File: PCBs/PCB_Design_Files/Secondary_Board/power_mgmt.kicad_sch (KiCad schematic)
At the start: 19 parts, among them Q3 MMBT3904, Q4 MMBT3904, U1 TPS61023DRLR, U2 TLV9101IDCKR

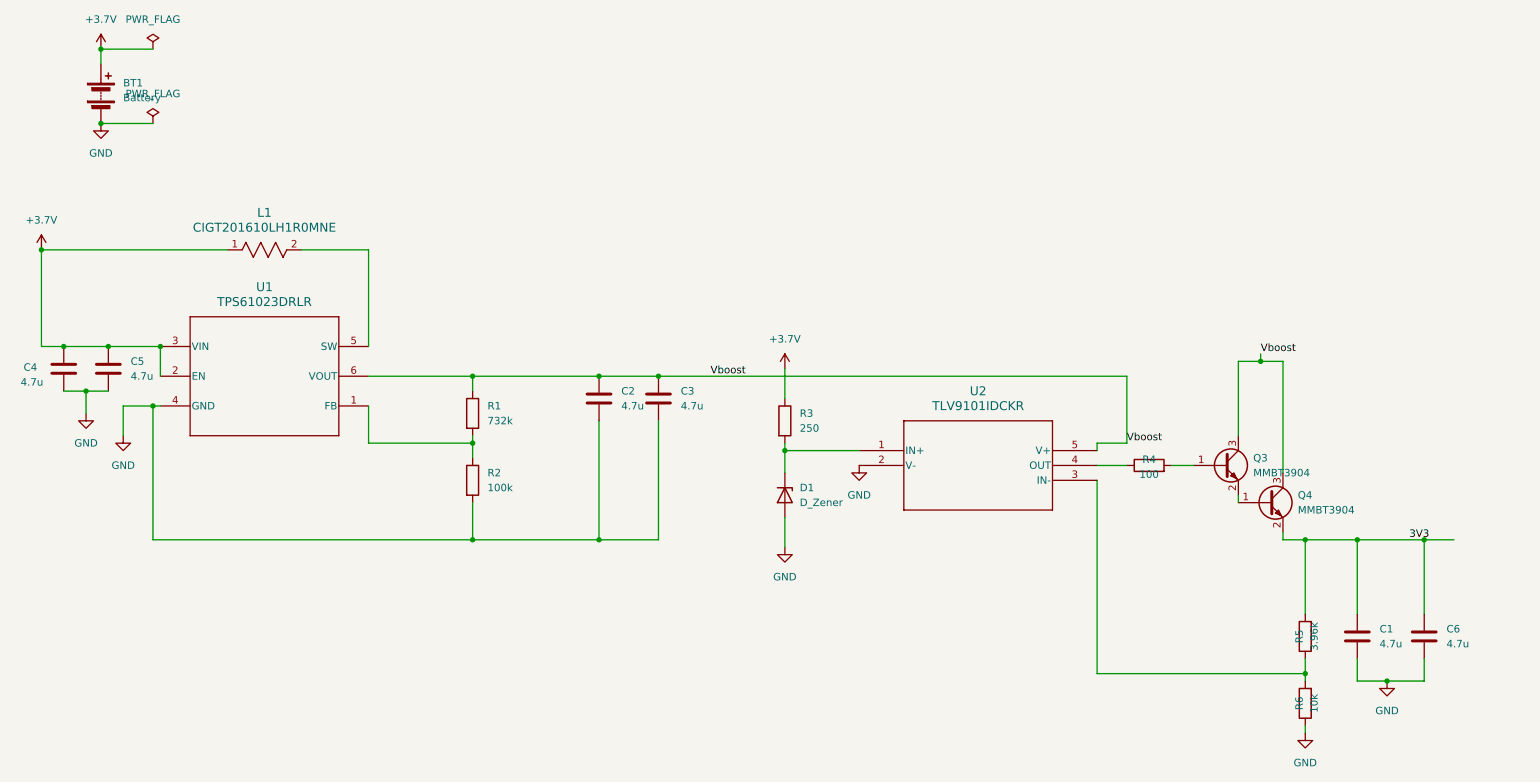
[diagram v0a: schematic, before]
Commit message: footprint update
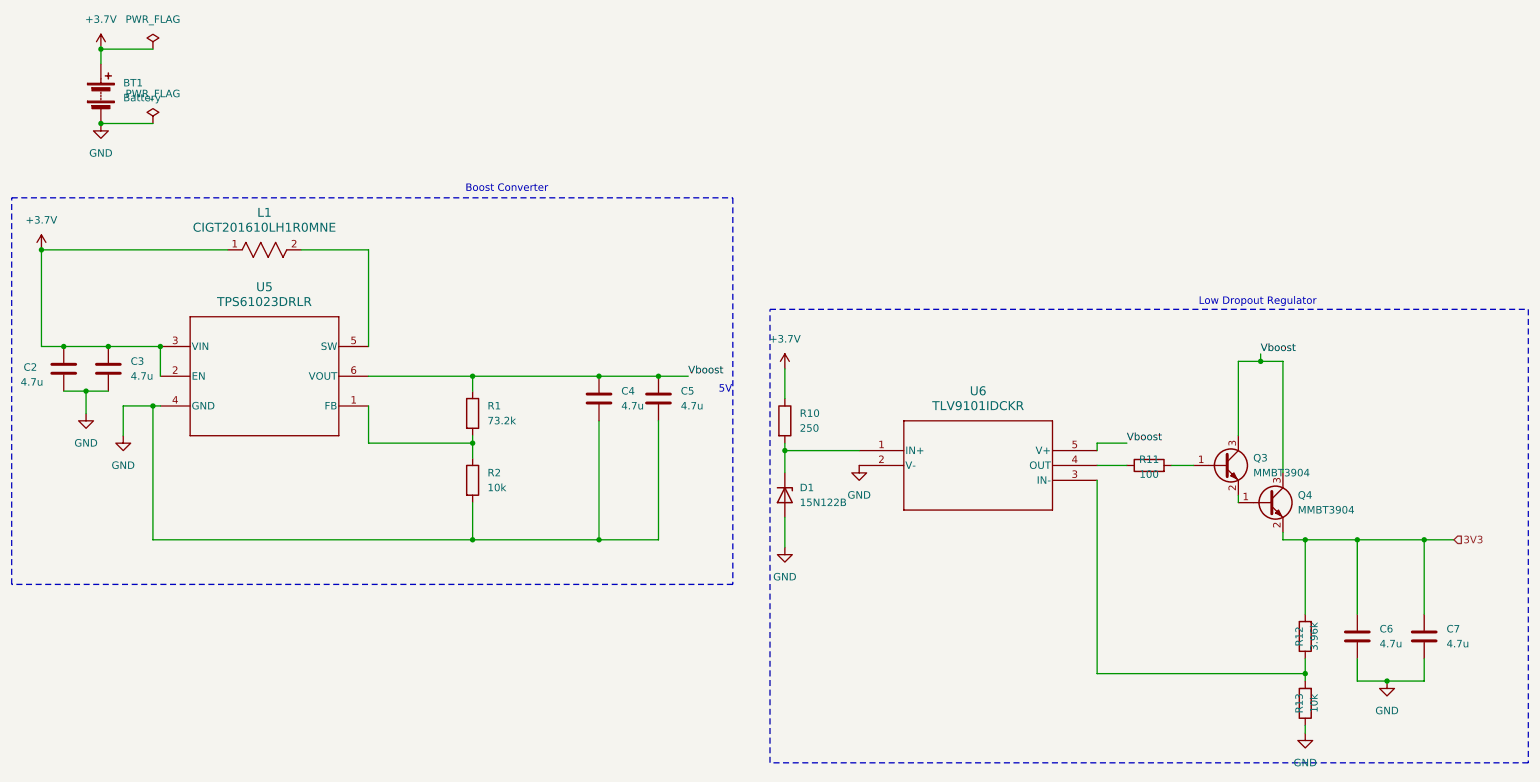
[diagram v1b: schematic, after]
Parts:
- BT1: footprint (none) -> Diode_THT:D_DO-35_SOD27_P7.62mm_Horizontal
- D1: value D_Zener -> 15N122B; footprint (none) -> Diode_THT:D_DO-35_SOD27_P7.62mm_Horizontal
- L1: footprint RES_CIGT201610_SAM -> Project Footprints:RES_CIGT201610_SAM
- Q3, Q4: footprint Package_TO_SOT_SMD:SOT-23 -> Project Footprints:SOT23_FAS
- R1: value 732k -> 73.2k; footprint Resistor_SMD:R_0201_0603Metric -> Project Footprints:0603_resistor
- R10: renamed from R3; footprint Resistor_SMD:R_0201_0603Metric -> Project Footprints:0603_resistor
- R11: renamed from R4; footprint Resistor_SMD:R_0201_0603Metric -> Project Footprints:0603_resistor
- R12: renamed from R5; footprint Resistor_SMD:R_0201_0603Metric -> Project Footprints:0603_resistor
- R13: renamed from R6; footprint Resistor_SMD:R_0201_0603Metric -> Project Footprints:0603_resistor
- R2: value 100k -> 10k; footprint (none) -> Project Footprints:0603_resistor
- U6: renamed from U2; footprint SC70-5_DCK_TEX -> Project Footprints:SC70-5_DCK_TEX
- renumbered C4 to C2, C5 to C3, C2 to C4, C3 to C5, C1 to C6, C6 to C7, U1 to U5
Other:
- note added: "5V"
- note added: "Boost Converter"
- note added: "Low Dropout Regulator"
